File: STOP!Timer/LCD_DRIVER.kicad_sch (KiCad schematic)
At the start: 5 parts, among them J2 Conn_01x16_Socket, Q1 2N2219, U4 PCF8574

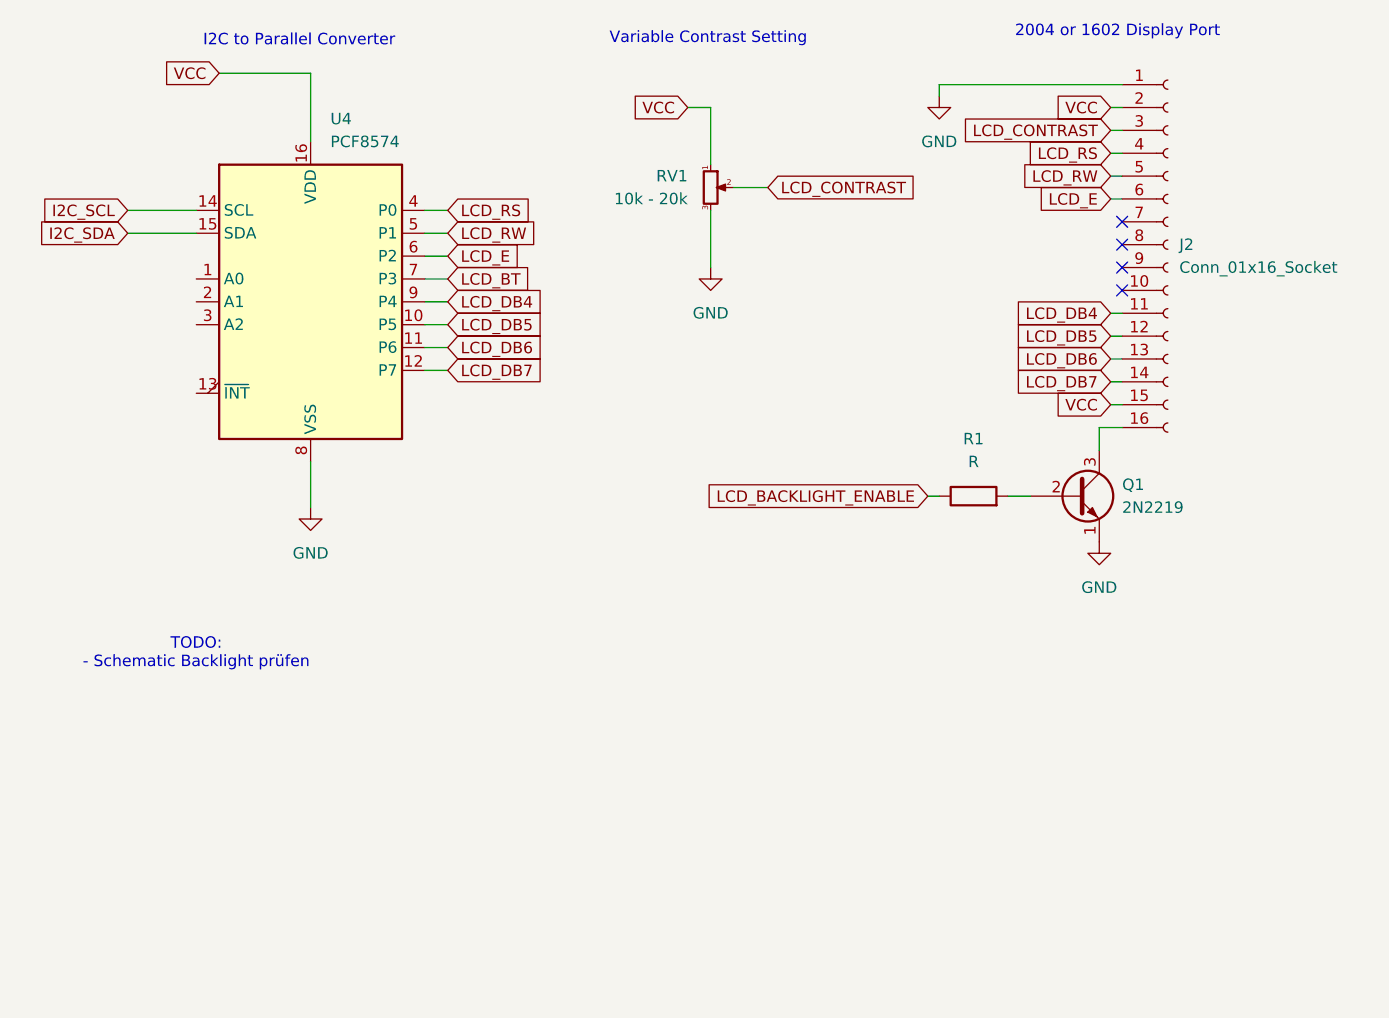
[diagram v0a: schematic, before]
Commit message: Update Schematic
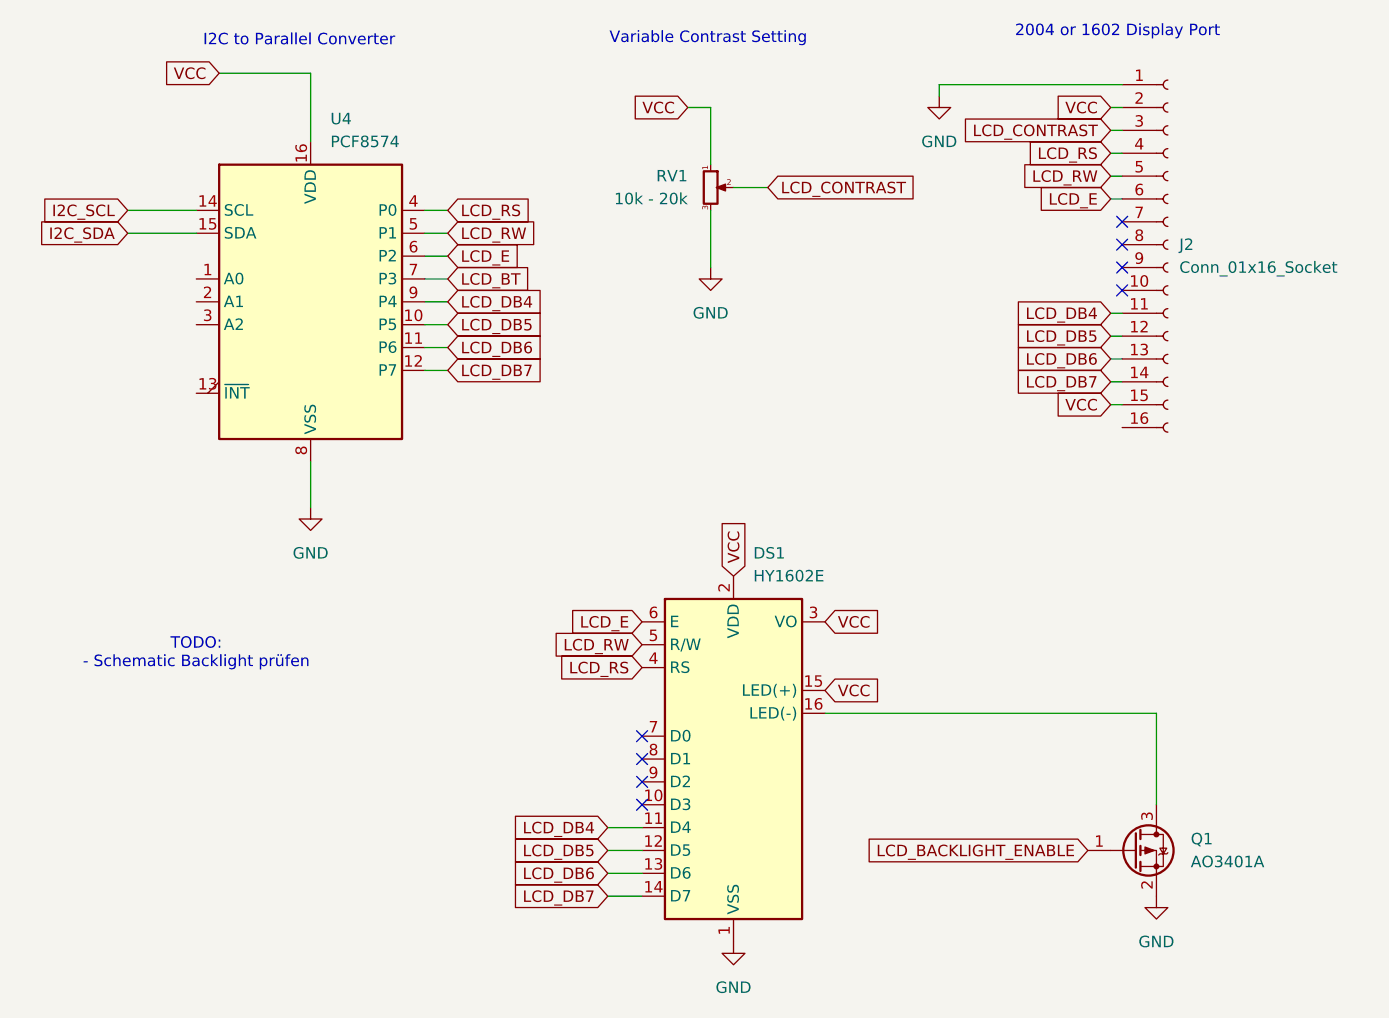
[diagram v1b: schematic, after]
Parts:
- removed Q1: 2N2219, Package_TO_SOT_THT:TO-39-3, symbol Transistor_BJT:2N2219
- removed R1: R, symbol Device:R
- added DS1: HY1602E, Display:WC1602A, symbol Display_Character:WC1602A
- added Q1: AO3401A, Package_TO_SOT_SMD:SOT-23, symbol Transistor_FET:AO3401A
- U4: footprint (none) -> Package_SO:SSOP-20_4.4x6.5mm_P0.65mm; JLC (none) -> C57790
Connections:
- net GND: now also DS1.1 (VSS), Q1.2 (S)
- net LCD_BACKLIGHT_ENABLE: now also Q1.1 (G)
- net LCD_DB4: now also DS1.11 (D4)
- net LCD_DB5: now also DS1.12 (D5)
- net LCD_DB6: now also DS1.13 (D6)
- net LCD_DB7: now also DS1.14 (D7)
- net LCD_E: now also DS1.6 (E)
- net LCD_RS: now also DS1.4 (RS)
- net LCD_RW: now also DS1.5 (R/W)
- net VCC: now also DS1.15 (LED(+)), DS1.2 (VDD), DS1.3 (VO)
- new net: DS1.16 (LED(-)), Q1.3 (D)
- no-connect marks 4 -> 8
